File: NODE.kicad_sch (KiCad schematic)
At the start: 76 parts, among them IC1 MP1584EN, J1 BUTTON, J2 ESP_PROG, J3 UART_SW, J4 CONNECTOR, J5 BATT, J6 ESP_ANT, J7 Conn_Coaxial, J8 LORA_ANT, J9 Conn_Coaxial, SW1 Reset, SW2 Boot, U1 AP1117-33, U2 ESP32-WROOM-32, U3 74HC14, U4 Ra-02, U5 MAX485E, U6 PCF8563T, Y1 32.768KHz

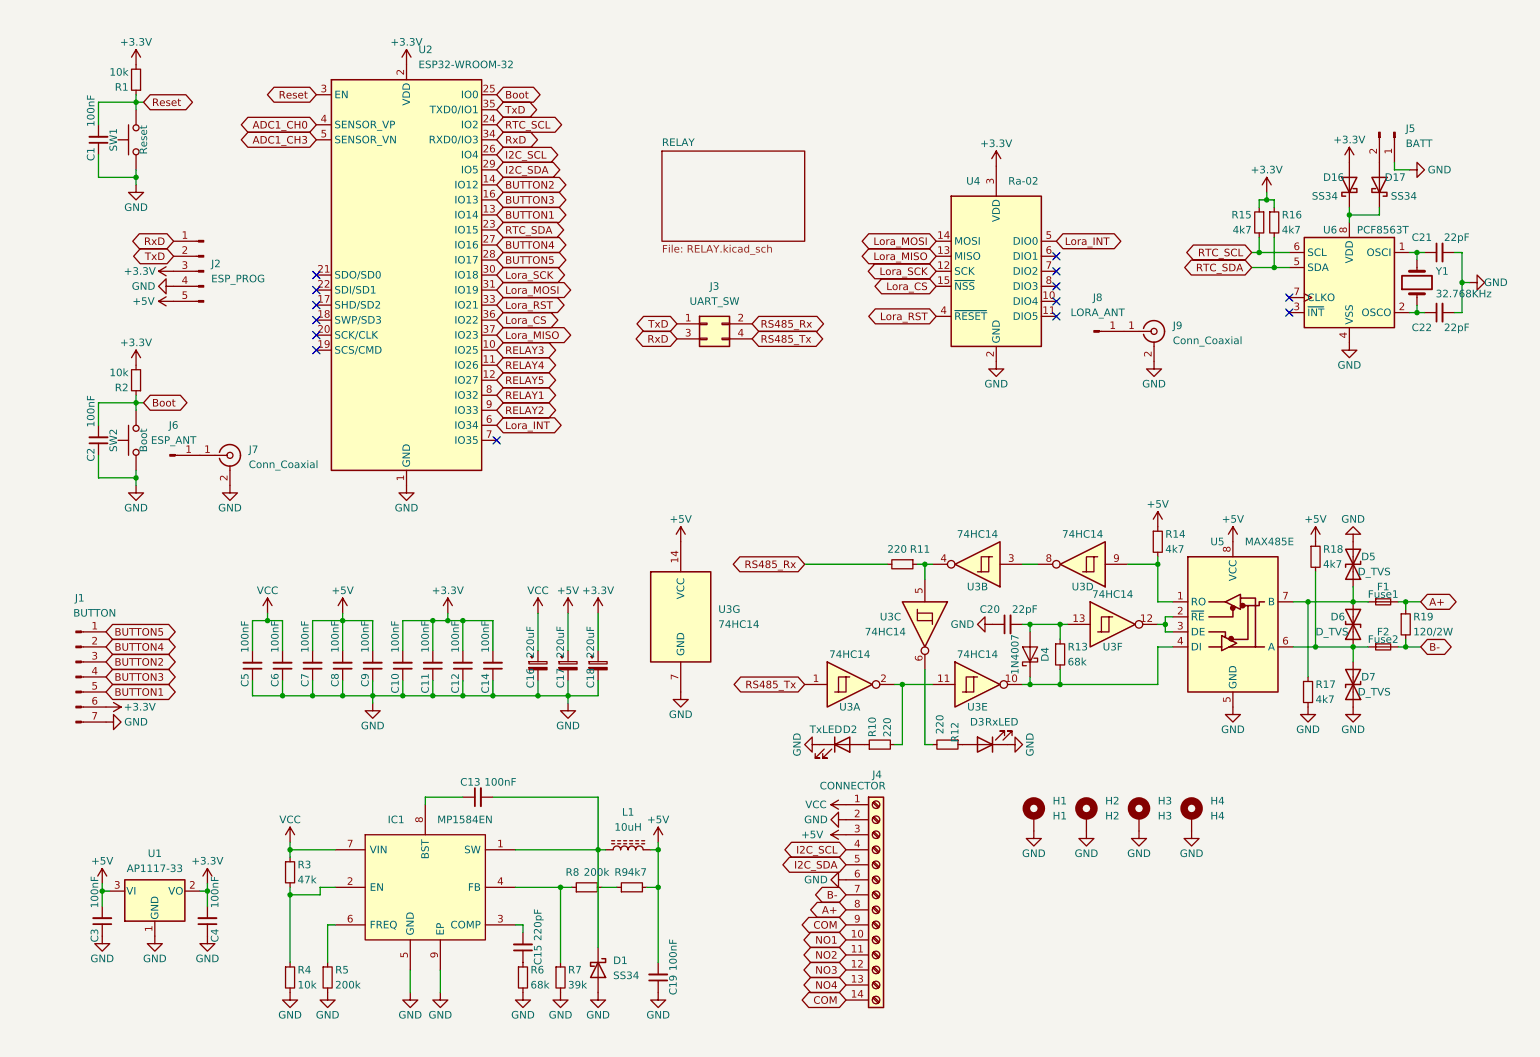
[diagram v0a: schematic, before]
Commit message: Add files via upload
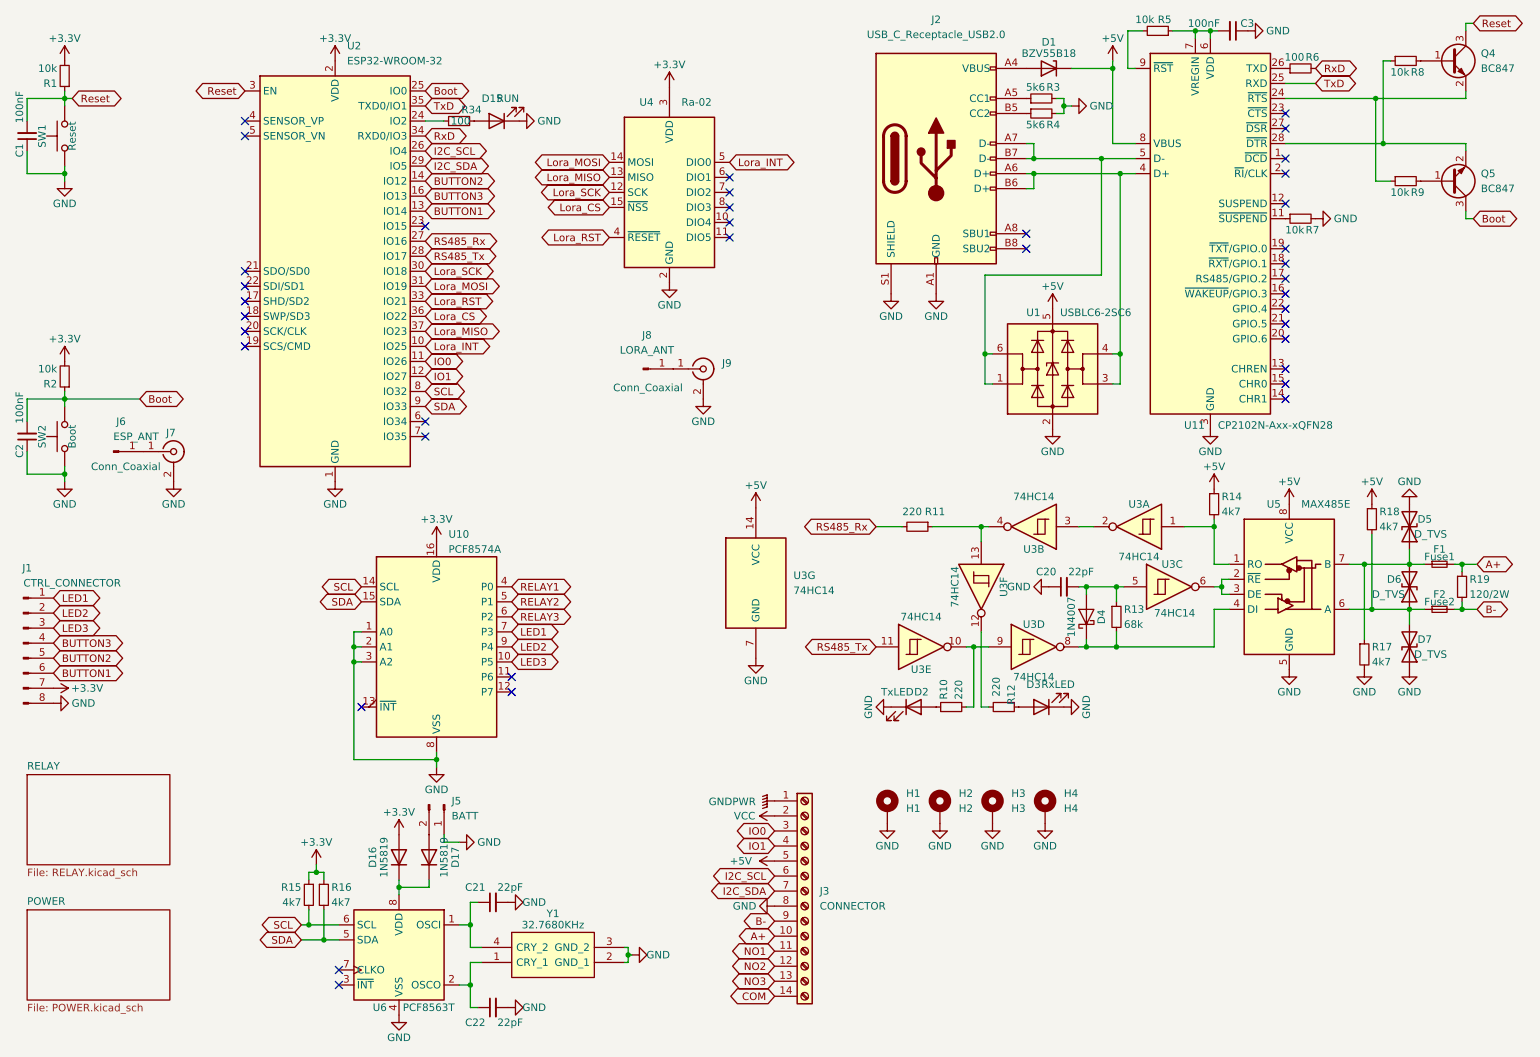
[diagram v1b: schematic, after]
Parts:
- removed C10, C11, C12, C13, C14, C19, C4, C5, C6, C7, C8, C9: 100nF, Capacitor_SMD:C_0603_1608Metric, symbol Device:C_Small
- removed C15: 220pF, Capacitor_SMD:C_0603_1608Metric, symbol Device:C_Small
- removed C16: 220uF, Capacitor_SMD:CP_Elec_8x10.5, symbol Device:C_Polarized_Small
- removed C17, C18: 220uF, Capacitor_SMD:CP_Elec_6.3x7.7, symbol Device:C_Polarized_Small
- removed D1, D16, D17: SS34, Diode_SMD:D_SMA, symbol Diode:CDBA340-HF
- removed IC1: MP1584EN, Package_SO:SOIC-8-1EP_3.9x4.9mm_P1.27mm_EP2.514x3.2mm_ThermalVias, symbol MP1584EN-LF-P:MP1584EN
- removed J1: BUTTON, XH_2.54mm_Conn:XH_7P_2.54mm_Horizontal, symbol Connector:Conn_01x07_Male
- removed J2: ESP_PROG, XH_2.54mm_Conn:XH_5P_2.54mm_Horizontal, symbol Connector:Conn_01x05_Male
- removed J3: UART_SW, Connector_PinHeader_2.54mm:PinHeader_2x02_P2.54mm_Vertical, symbol Connector_Generic:Conn_02x02_Odd_Even
- removed J4: CONNECTOR, TerminalBlock_Phoenix:TerminalBlock_Phoenix_MKDS-1,5-14-5.08_1x14_P5.08mm_Horizontal, symbol Connector:Screw_Terminal_01x14
- removed L1: 10uH, Inductor_SMD:L_Abracon_ASPI-0630LR, symbol Device:L_Ferrite
- removed U1: AP1117-33, Package_TO_SOT_SMD:SOT-223-3_TabPin2, symbol Regulator_Linear:AP1117-33
- removed Y1: 32.768KHz, MC-306:MC306327680KE3ROHS, symbol Device:Crystal
- added D1: BZV55B18, Diode_SMD:D_MiniMELF, symbol Diode:BZV55B18
- added D15: RUN, LED_SMD:LED_0603_1608Metric, symbol Device:LED
- added D16, D17: 1N5819, Diode_SMD:D_SOD-123, symbol Diode:1N4148W
- added J1: CTRL_CONNECTOR, XH_2.54mm_Conn:XH_8P_2.54mm_Vertical, symbol Connector:Conn_01x08_Male
- added J2: USB_C_Receptacle_USB2.0, Connector_USB:USB_C_Receptacle_HRO_TYPE-C-31-M-12, symbol Connector:USB_C_Receptacle_USB2.0
- added J3: CONNECTOR, TerminalBlock_Phoenix:TerminalBlock_Phoenix_MKDS-1,5-14-5.08_1x14_P5.08mm_Horizontal, symbol Connector:Screw_Terminal_01x14
- added Q4, Q5: BC847, Package_TO_SOT_SMD:SOT-23, symbol Transistor_BJT:BC847
- added R34: 100, Resistor_SMD:R_0603_1608Metric, symbol Device:R_Small
- added U1: USBLC6-2SC6, Package_TO_SOT_SMD:SOT-23-6, symbol Power_Protection:USBLC6-2SC6
- added U10: PCF8574A, Package_SO:SOIC-16W_7.5x10.3mm_P1.27mm, symbol Interface_Expansion:PCF8574A
- added U11: CP2102N-Axx-xQFN28, Package_DFN_QFN:QFN-28-1EP_5x5mm_P0.5mm_EP3.35x3.35mm, symbol Interface_USB:CP2102N-Axx-xQFN28
- added Y1: 32.7680KHz, MC-306:MC306327680KE3ROHS, symbol MC-306_32.7680K-E3_ROHS:MC-306_32.7680K-E3_ROHS
- R3: value 47k -> 5k6
- R4: value 10k -> 5k6
- R5, R8: value 200k -> 10k
- R6: value 68k -> 100
- R7: value 39k -> 10k
- R9: value 4k7 -> 10k
- U5: footprint Package_SO:SOIC-8-1EP_3.9x4.9mm_P1.27mm_EP2.41x3.3mm_ThermalVias -> Package_SO:SOIC-8_3.9x4.9mm_P1.27mm
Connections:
- net BUTTON4 is gone; now on net RS485_Rx: U2.27 (IO16)
- net BUTTON5 is gone; now on net RS485_Tx: U2.28 (IO17)
- net +3.3V: now also D16.2 (A), J1.7 (Pin_7), U10.16 (VDD)
- net +5V: now also D1.1 (K), J3.5 (Pin_5), U1.5 (VBUS), U11.8 (VBUS); no longer C3.2, R9.2
- net A+: now also J3.10 (Pin_10)
- net B-: now also J3.9 (Pin_9)
- net BUTTON1: now also J1.6 (Pin_6)
- net BUTTON2: now also J1.5 (Pin_5)
- net BUTTON3: now also J1.4 (Pin_4)
- net Boot: now also Q5.3 (C)
- net COM: now also J3.14 (Pin_14)
- net GND: now also R3.2, D15.1 (K), J1.8 (Pin_8), J2.A1 (GND), J2.A12 (GND), J2.B1 (GND), J2.B12 (GND), J2.S1 (SHIELD), J3.8 (Pin_8), U1.2 (GND), U10.1 (A0), U10.2 (A1), U10.3 (A2), U10.8 (VSS), U11.29 (GND), U11.3 (GND), Y1.2 (GND_1), Y1.3 (GND_2); no longer R5.2, R6.2
- net I2C_SCL: now also J3.6 (Pin_6)
- net I2C_SDA: now also J3.7 (Pin_7)
- net Lora_INT: now also U2.10 (IO25); no longer U2.6 (IO34)
- net NO1: now also J3.11 (Pin_11)
- net NO2: now also J3.12 (Pin_12)
- net NO3: now also J3.13 (Pin_13)
- net RELAY1: now also U10.4 (P0); no longer U2.8 (IO32)
- net RELAY2: now also U10.5 (P1); no longer U2.9 (IO33)
- net RELAY3: now also U10.6 (P2); no longer U2.10 (IO25)
- net RS485_Tx: now also U3.11; no longer U3.1
- net Reset: now also Q4.3 (C)
- net RxD: now also R6.2
- net TxD: now also U11.25 (RXD)
- net VCC: now also J3.2 (Pin_2); no longer R3.1
- net at C20.2, D4.2 (A), R13.1: now also U3.5; no longer U3.13
- net at R4.1: now also J2.B5 (CC2); no longer R3.2
- net at U6.8 (VDD): now also D16.1 (K), D17.1 (K)
- net at C21.1, U6.1 (OSCI): now also Y1.4 (CRY_2)
- net at R5.1: now also C3.2, U11.6 (VDD), U11.7 (VREGIN)
- net at C22.1, U6.2 (OSCO): now also Y1.1 (CRY_1)
- net at R8.1: now also Q5.2 (E), U11.28 (~{DTR}); no longer R7.1
- net at R12.2: now also U3.12; no longer U3.6
- net at D4.1 (K), R13.2, U5.4 (DI): now also U3.8; no longer U3.10
- net at R14.2, U5.1 (RO): now also U3.1; no longer U3.9
- net at U5.2 (~{RE}), U5.3 (DE): now also U3.6; no longer U3.12
- net at R11.1, U3.4: now also U3.13; no longer U3.5
- net at U3.3: now also U3.2; no longer U3.8
- net at R9.1: now also Q4.2 (E), U11.24 (~{RTS}); no longer R8.2
- net at J5.2 (Pin_2): now also D17.2 (A)
- net at R6.1: now also U11.26 (TXD)
- net ADC1_CH0: no longer names the net of U2.4 (SENSOR_VP)
- net ADC1_CH3: no longer names the net of U2.5 (SENSOR_VN)
- net RELAY4 renamed IO0
- net IO0: now also J3.3 (Pin_3)
- net RELAY5 renamed IO1
- net IO1: now also J3.4 (Pin_4)
- net RTC_SCL renamed SCL
- net SCL: now also U2.8 (IO32), U10.14 (SCL); no longer U2.24 (IO2)
- net RTC_SDA renamed SDA
- net SDA: now also U2.9 (IO33), U10.15 (SDA); no longer U2.23 (IO15)
- new net: Q5.1 (B), R9.2
- new net: R7.1, U11.11 (~{SUSPEND})
- new net: J2.A6 (D+), J2.B6 (D+), U1.3 (I/O2), U1.4 (I/O2), U11.4 (D+)
- new net: J2.A7 (D-), J2.B7 (D-), U1.1 (I/O1), U1.6 (I/O1), U11.5 (D-)
- new net: R5.2, U11.9 (~{RST})
- new net: D15.2 (A), R34.2
- new net: J2.A5 (CC1), R3.1
- new net: R34.1, U2.24 (IO2)
- new net: R10.2, U3.10, U3.9
- new net: Q4.1 (B), R8.2
- new net: D1.2 (A), J2.A4 (VBUS), J2.A9 (VBUS), J2.B4 (VBUS), J2.B9 (VBUS)
- new net GNDPWR: J3.1 (Pin_1)
- new net LED1: J1.1 (Pin_1), U10.7 (P3)
- new net LED2: J1.2 (Pin_2), U10.9 (P4)
- new net LED3: J1.3 (Pin_3), U10.10 (P5)
- no-connect marks 14 -> 38
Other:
- added sheet POWER (POWER.kicad_sch)
- moved on the sheet: C1, C2, C20, C21, C22, D2, D3, D4, D5, D6, D7, F1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
